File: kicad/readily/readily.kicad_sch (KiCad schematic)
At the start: 29 parts, among them J1 Conn_01x09_Socket, J3 USB_C_Receptacle_USB2.0_16P, J4 Conn_01x03, SW2 SW_SPST, SW3 SW_SPST, U1 ESP32-S3-WROOM-1, U2 BQ24040DSQR, U3 TPD2EUSB30, U4 TLV75533PDRV, U5 ED08905M-FE15C7_0-C10-2053

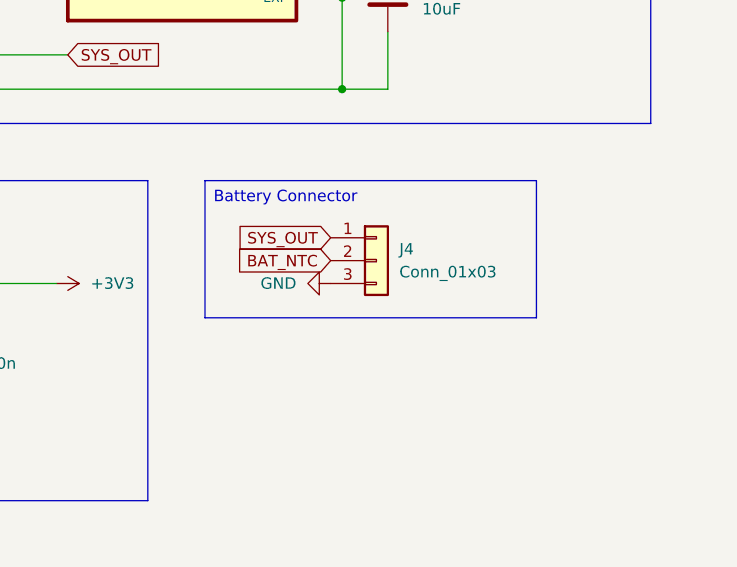
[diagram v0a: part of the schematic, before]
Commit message: feat: version 1.0 of the pcb
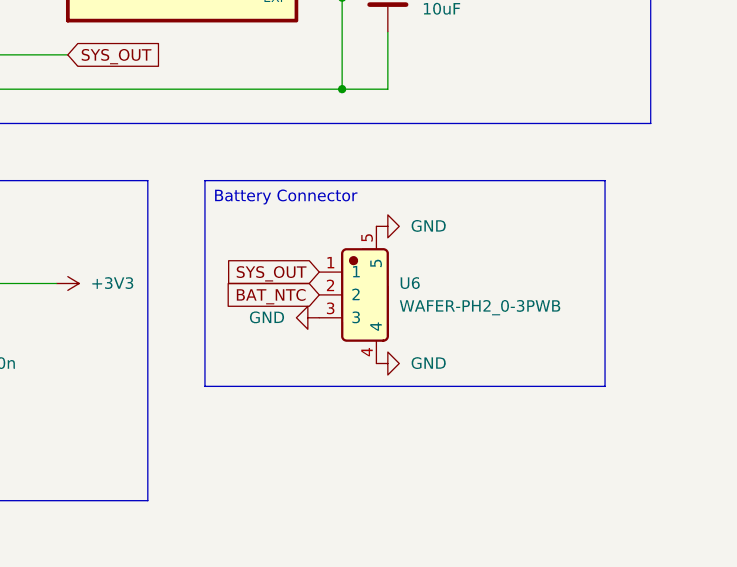
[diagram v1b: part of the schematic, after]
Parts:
- removed J4: Conn_01x03, JST_PH_B3B-PH-K_1x03_P2.00mm_Vertical, symbol Connector_Generic:Conn_01x03
- added U6: WAFER-PH2_0-3PWB, JLCImport:WAFER-PH2_0-3PWB, symbol ED08905M-FE15C7.0-C10-2053:WAFER-PH2_0-3PWB
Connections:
- net BAT_NTC: now also U6.2
- net GND: now also U6.3, U6.4, U6.5
- net SYS_OUT: now also U6.1
